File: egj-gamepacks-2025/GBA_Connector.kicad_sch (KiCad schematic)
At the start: 7 parts, among them J5 GameBoy_GamePak_AGB-002, U10 SP3012-06UTG, U15 SP3012-06UTG, U6 SP3012-06UTG, U7 SP3012-06UTG, U8 SP3012-06UTG, U9 SP3012-06UTG

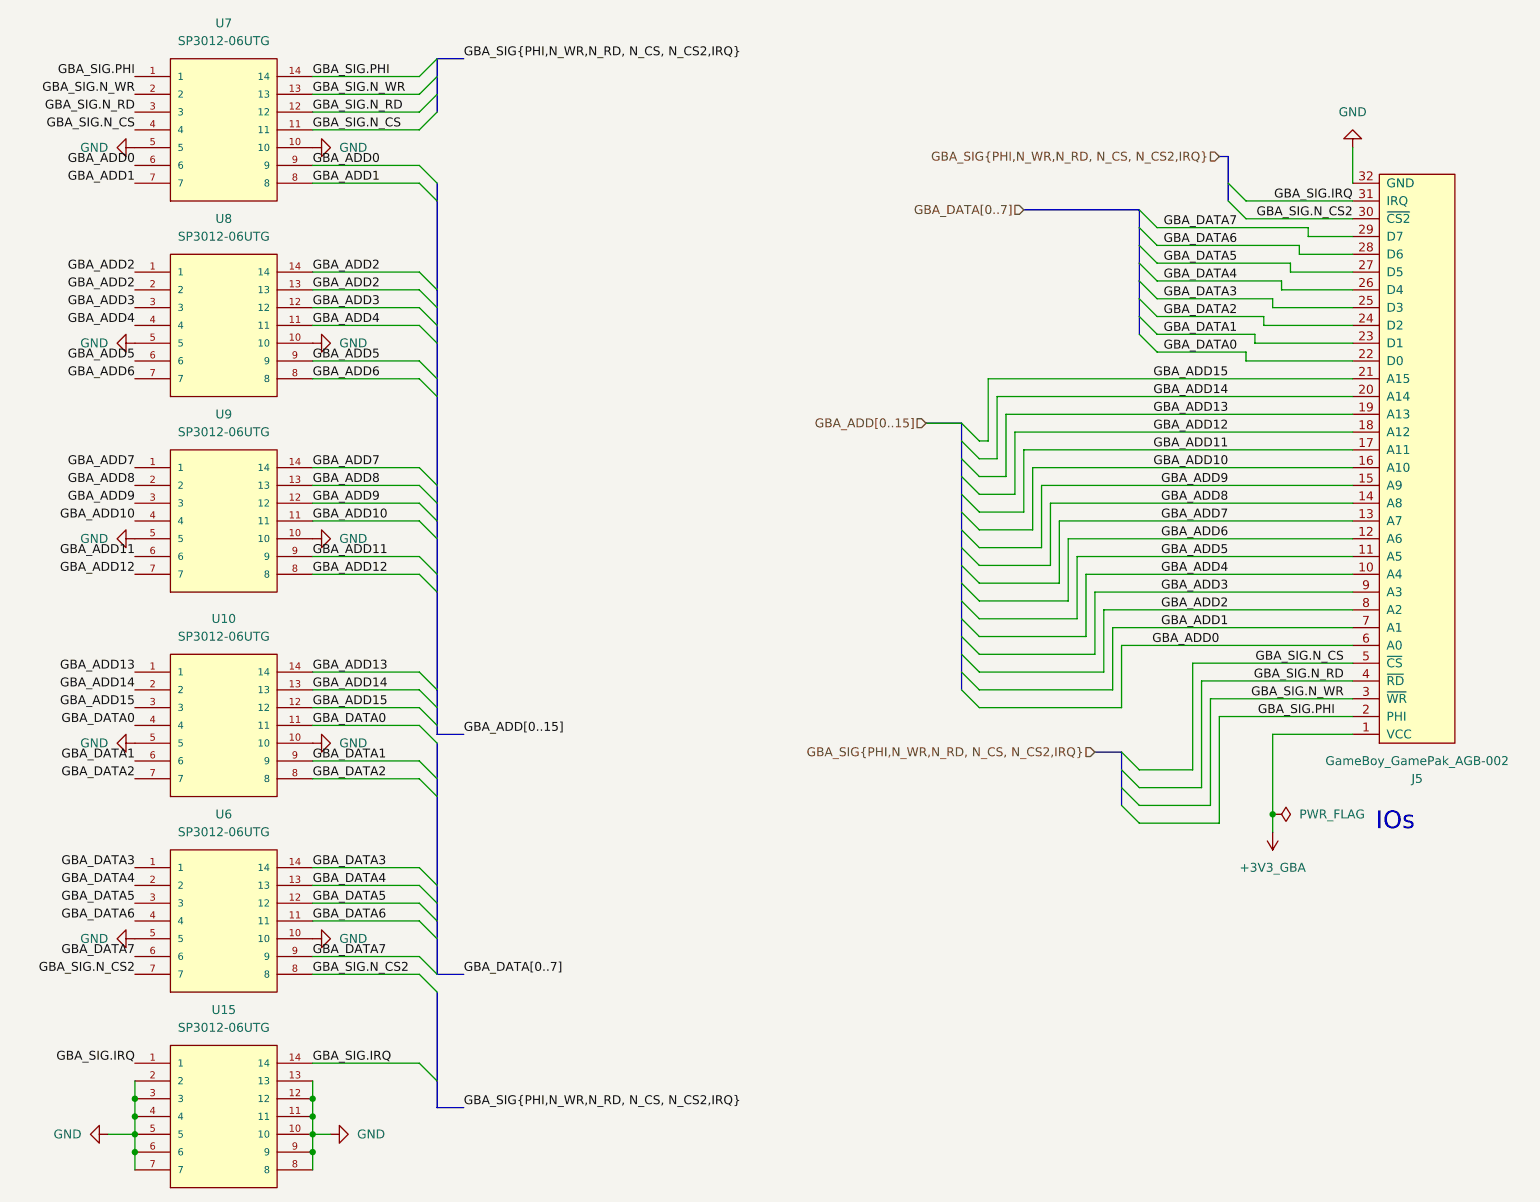
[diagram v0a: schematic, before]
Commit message: UPDATE: sync local schematic and board work
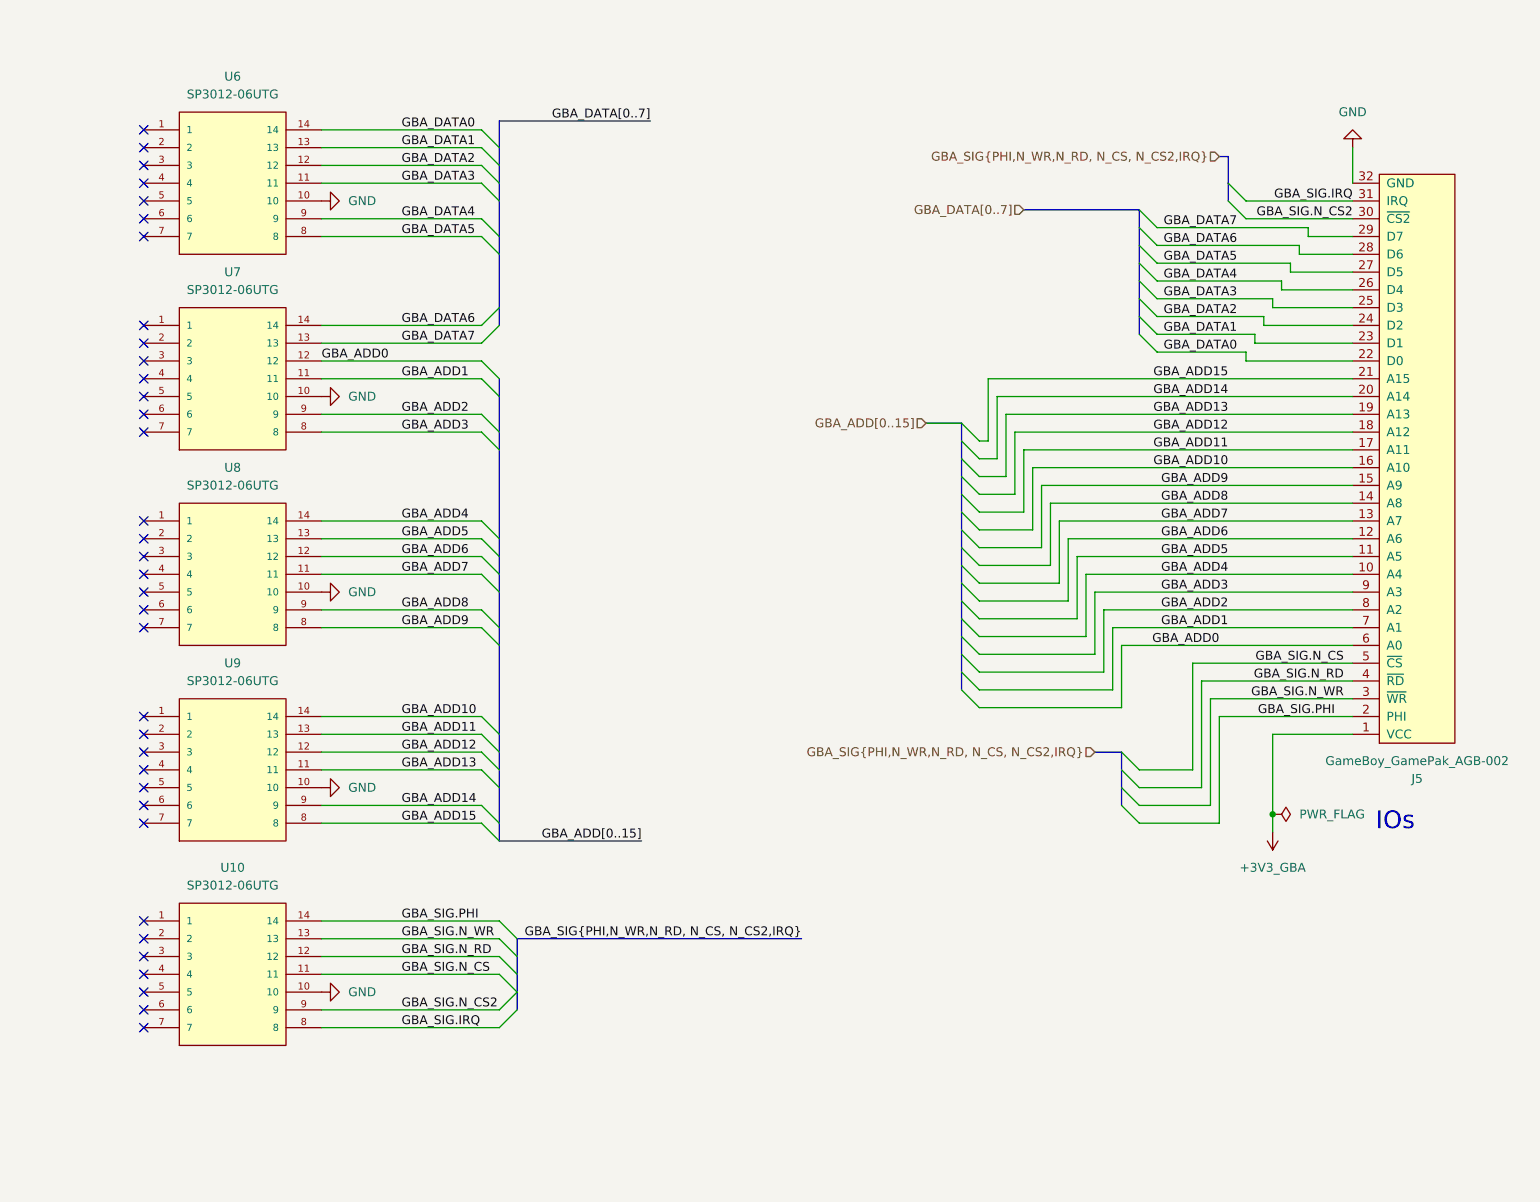
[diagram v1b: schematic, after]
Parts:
- removed U15: SP3012-06UTG, Package_DFN_QFN:DFN-14_1.35x3.5mm_P0.5mm, symbol SP3012-06UTG:SP3012-06UTG
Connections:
- net GBA_ADD0: now also U7.12; no longer U7.6, U7.9
- net GBA_ADD1: now also U7.11; no longer U7.7, U7.8
- net GBA_ADD10: now also U9.14; no longer U9.11, U9.4
- net GBA_ADD11: now also U9.13; no longer U9.6, U9.9
- net GBA_ADD12: now also U9.12; no longer U9.7, U9.8
- net GBA_ADD13: now also U9.11; no longer U10.1, U10.14
- net GBA_ADD14: now also U9.9; no longer U10.13, U10.2
- net GBA_ADD15: now also U9.8; no longer U10.12, U10.3
- net GBA_ADD2: now also U7.9; no longer U8.1, U8.13, U8.14, U8.2
- net GBA_ADD3: now also U7.8; no longer U8.12, U8.3
- net GBA_ADD4: now also U8.14; no longer U8.11, U8.4
- net GBA_ADD5: now also U8.13; no longer U8.6, U8.9
- net GBA_ADD6: now also U8.12; no longer U8.7, U8.8
- net GBA_ADD7: now also U8.11; no longer U9.1, U9.14
- net GBA_ADD8: now also U8.9; no longer U9.13, U9.2
- net GBA_ADD9: now also U8.8; no longer U9.12, U9.3
- net GBA_DATA0: now also U6.14; no longer U10.11, U10.4
- net GBA_DATA1: now also U6.13; no longer U10.6, U10.9
- net GBA_DATA2: now also U6.12; no longer U10.7, U10.8
- net GBA_DATA3: now also U6.11; no longer U6.1, U6.14
- net GBA_DATA4: now also U6.9; no longer U6.13, U6.2
- net GBA_DATA5: now also U6.8; no longer U6.12, U6.3
- net GBA_DATA6: now also U7.14; no longer U6.11, U6.4
- net GBA_DATA7: now also U7.13; no longer U6.6, U6.9
- net GBA_SIG.IRQ: now also U10.8
- net GBA_SIG.N_CS: now also U10.11; no longer U7.11, U7.4
- net GBA_SIG.N_CS2: now also U10.9; no longer U6.7, U6.8
- net GBA_SIG.N_RD: now also U10.12; no longer U7.12, U7.3
- net GBA_SIG.N_WR: now also U10.13; no longer U7.13, U7.2
- net GBA_SIG.PHI: now also U10.14; no longer U7.1, U7.14
- net GND: no longer U10.5, U6.5, U7.5, U8.5, U9.5
- no-connect marks 0 -> 35
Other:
- moved on the sheet: U10, U6, U7, U8, U9
